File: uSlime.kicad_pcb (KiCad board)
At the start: 2 copper layers, 30 x 30 mm, 30 parts, among them J1 USB_B_Micro, U1 ESP32-C6-MINI-1, U2 S2B-PH-K-S-GW, U3 AP2112K-3.3TRG1, U4 MCP73831T-2ACI/OT, U5 BNO085, U6 MSK-12C02_SMD_SPDT_SWITCH, Y1 32.768

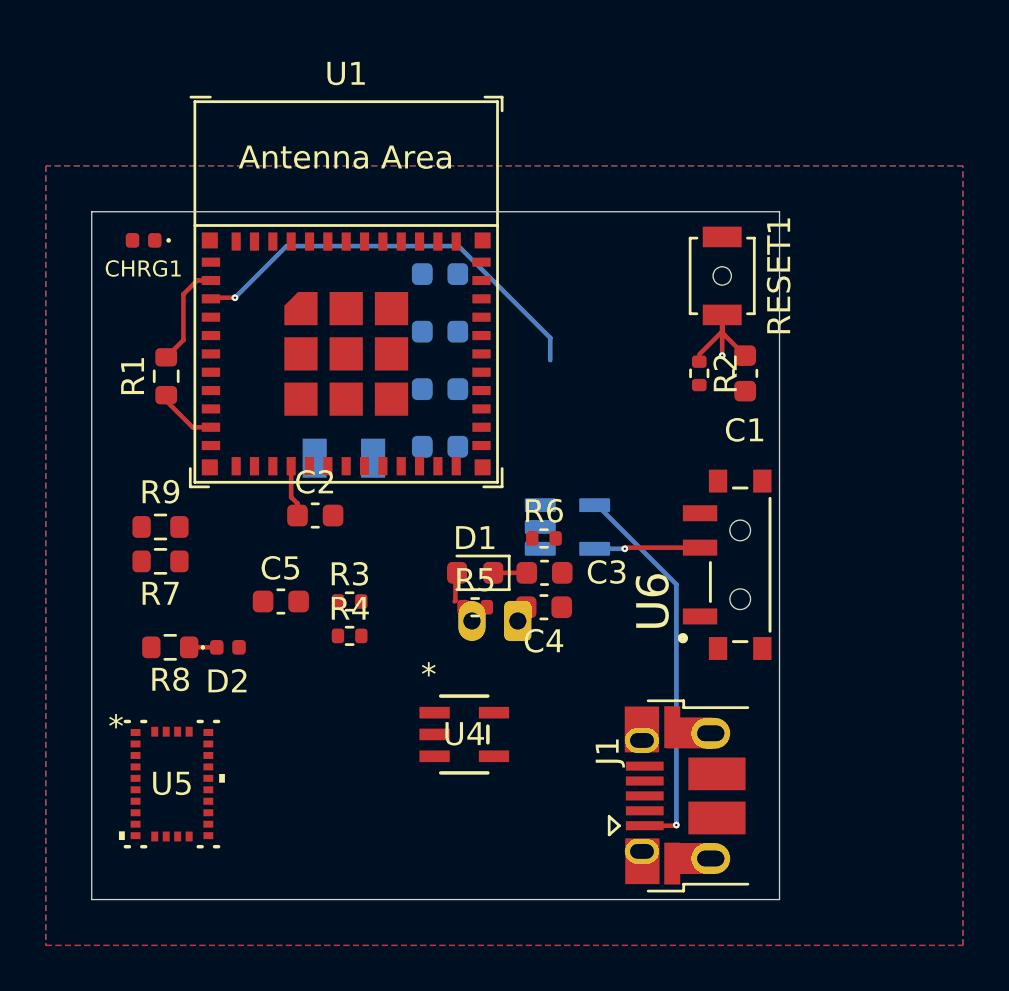
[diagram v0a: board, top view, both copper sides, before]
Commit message: PCB Smol Time
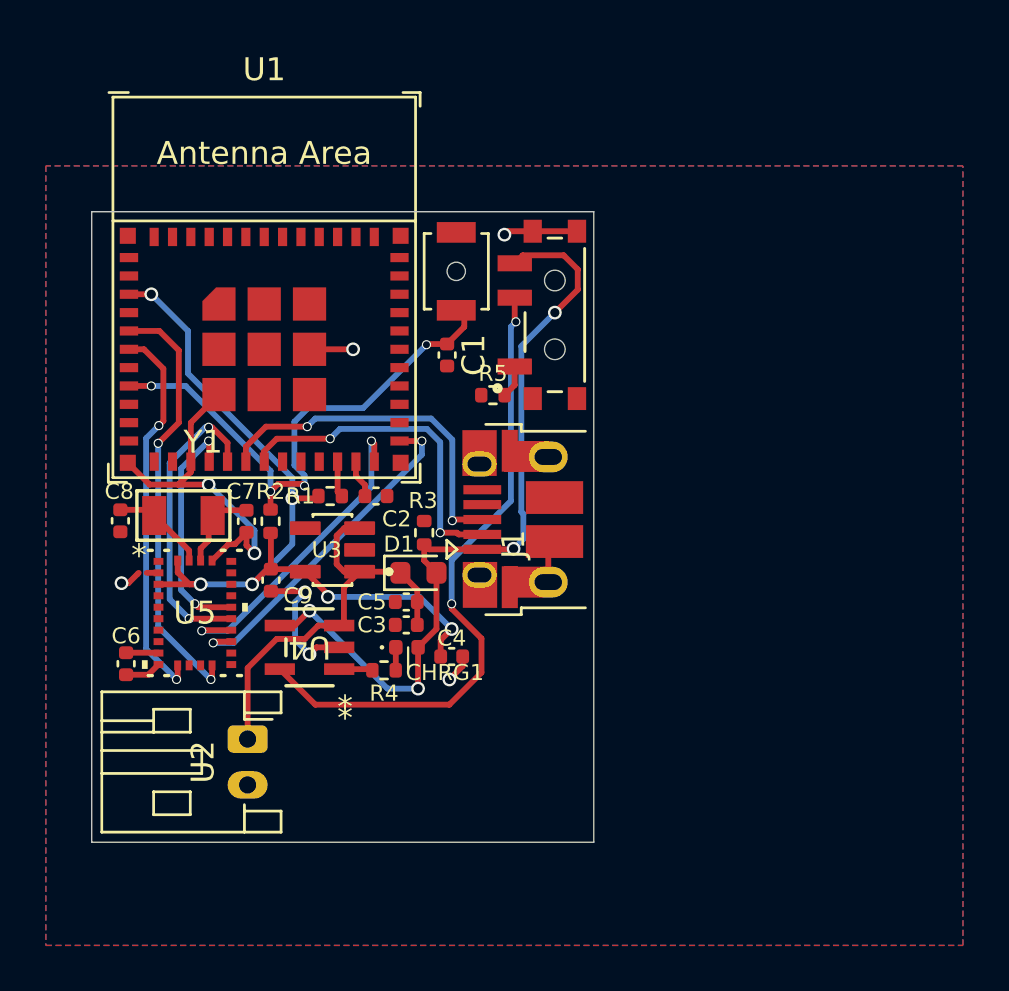
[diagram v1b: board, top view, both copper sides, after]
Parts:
- removed D2: LED, LED_SMD:LED_0402_1005Metric
- removed R6: 100KOHM-0402T-1/16W-1%, Resistor_SMD:R_0402_1005Metric
- removed R7: 100K, Resistor_SMD:R_0603_1608Metric
- removed R8: 1k, Resistor_SMD:R_0603_1608Metric
- removed R9: 4.7k, Resistor_SMD:R_0603_1608Metric
- C1, C2, C3, C4, C5: footprint Capacitor_SMD:C_0603_1608Metric -> Capacitor_SMD:C_0402_1005Metric
- C6, C7, C8, C9: footprint Capacitor_SMD:C_0603_1608Metric -> Capacitor_SMD:C_0402_1005Metric; moved to F.Cu
- R1: value 100KOHM-0603-1/10W-1% -> 100KOHM-0402T-1/16W-1%; footprint Resistor_SMD:R_0603_1608Metric -> Resistor_SMD:R_0402_1005Metric
- U2, U3, Y1: moved to F.Cu
- moved C6 21.8 mm to (102.2, 109.1), turned to 90 degrees
- moved CHRG1 21.1 mm to (114.4, 108.3), turned to 0 degrees
- moved R2 19.8 mm to (108.5, 102.8)
- moved C8 15.1 mm to (101.9, 102.8), turned to 90 degrees
- moved J1 14.0 mm to (119.5, 102.8)
- moved U6 13.6 mm to (120.8, 93.8)
- moved C1 13.0 mm to (116.2, 95.6)
- moved U2 12.9 mm to (107.5, 112.3), turned to -90 degrees
- moved C7 11.8 mm to (107.4, 102.8), turned to 90 degrees
- moved RESET1 11.6 mm to (116.5, 92.0)
- moved U3 10.3 mm to (111.2, 104.1), turned to 180 degrees
- moved C9 9.40 mm to (108.5, 105.4), turned to -90 degrees
- moved R5 9.28 mm to (118.2, 97.3)
- moved R1 8.86 mm to (111.0, 101.8), turned to 180 degrees
- moved U4 7.75 mm to (110.2, 108.3), turned to 180 degrees
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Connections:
- R5 pad 2: unconnected-(R5-Pad2) -> Net-(R5-Pad2)
- U1 pad 5: /ESP32-C6FH4/IO2 -> BNO_INT
- U1 pad 6: /ESP32-C6FH4/IO3 -> BNO_RST
- U5 pad 14: unconnected-(U5-H_INTN-Pad14) -> BNO_INT
- U6 pad L1: unconnected-(U6-PadL1) -> VBUS
- U6 pad L2: unconnected-(U6-PadL2) -> Net-(R5-Pad2)
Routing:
- net GND: track 0.00 -> 32.8 mm, vias 0 -> 8
- net Net-(U4-PROG): track 0.00 -> 28.1 mm, vias 1 -> 2
- net BNO_INT: track 0.00 -> 18.8 mm, vias 0 -> 2
- net /ESP32-C6FH4/ESP_EN: track 6.10 -> 23.7 mm, vias 1 -> 4
- net BNO_RST: track 0.00 -> 16.9 mm, vias 0 -> 2
- net VBUS: track 18.3 -> 35.1 mm, vias 1 -> 4
- net VBAT: track 1.95 -> 18.5 mm
- net D- N: track 0.00 -> 15.4 mm, vias 0 -> 2
- net BNO_MOSI: track 0.00 -> 14.9 mm, vias 0 -> 2
- net D+ P: track 0.00 -> 14.6 mm, vias 0 -> 2
- net BNO_CS: track 0.00 -> 14.3 mm, vias 0 -> 2
- net +3.3V: track 22.9 -> 37.0 mm, vias 1 -> 6
- net BNO_SCL: track 0.00 -> 13.3 mm, vias 0 -> 2
- net BNO_SDA: track 0.00 -> 10.4 mm, vias 0 -> 2
- net (no net): track 4.51 -> 0.00 mm
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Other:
- board size 30 x 30 mm -> 21.9 x 27.5 mm
